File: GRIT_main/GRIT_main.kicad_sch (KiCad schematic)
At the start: 22 parts, among them J1 Raspberry_Pi_4, M1 Motor_DC, M2 Motor_DC, M3 Motor_DC, M4 Motor_DC

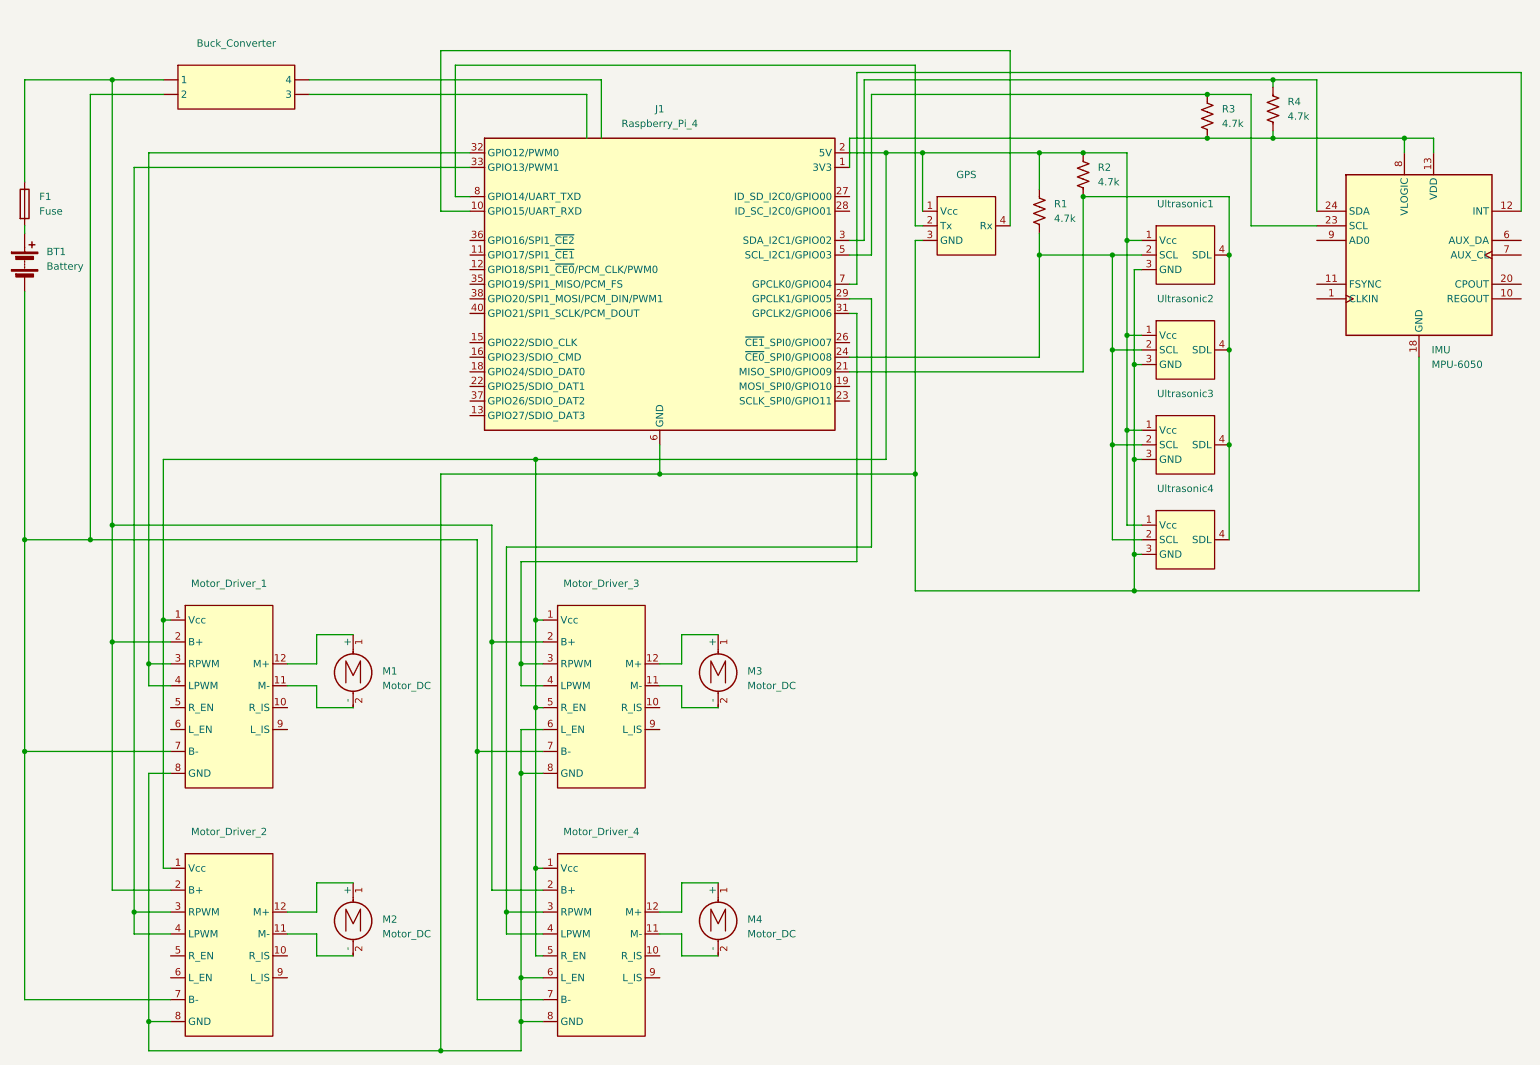
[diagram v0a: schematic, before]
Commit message: Updated Schematic
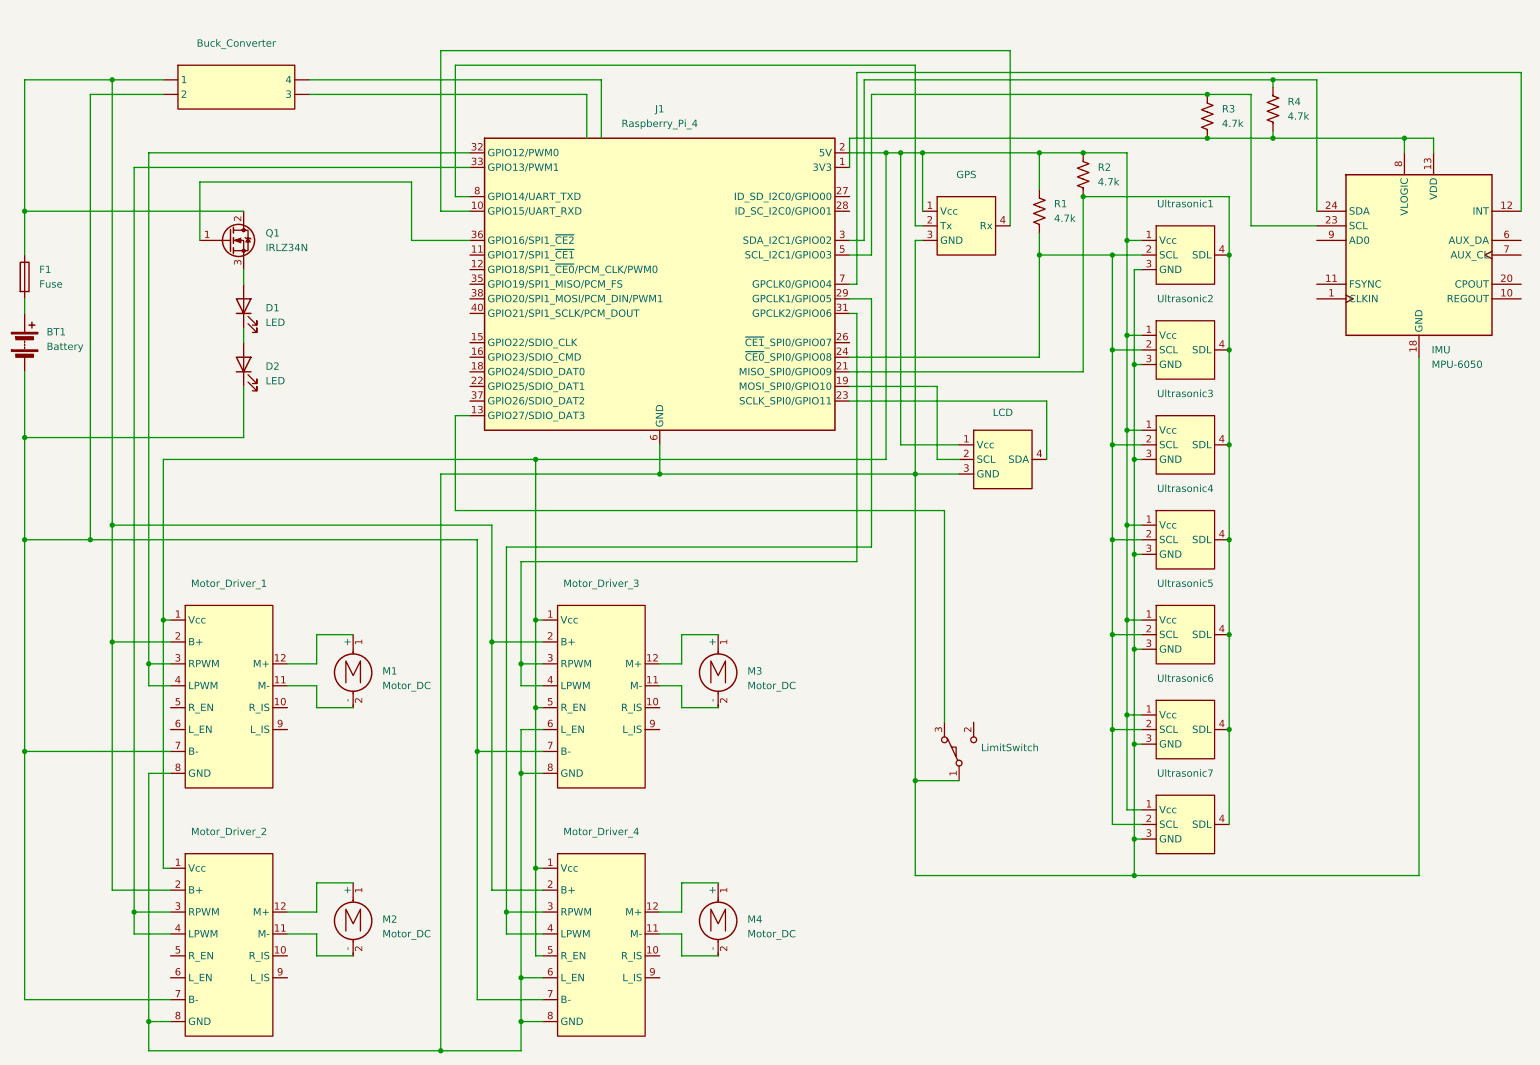
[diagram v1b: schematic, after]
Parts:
- added D1, D2: LED, symbol Device:LED
- added LCD: ~, symbol Custom_Symbols:I2C_LCD_Screen
- added LimitSwitch: ~, symbol Switch:SW_SPDT_XKB_DMx-xxxx-1
- added Q1: IRLZ34N, Package_TO_SOT_THT:TO-220-3_Vertical, symbol Transistor_FET:IRLZ34N
- added Ultrasonic5, Ultrasonic6, Ultrasonic7: ~, symbol Custom_Symbols:I2C_Ultrasonic_Sensor
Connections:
- net at GPS.3 (GND), IMU.18 (GND), J1.14 (GND)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: now also LCD.3 (GND), LimitSwitch.1 (A), Ultrasonic5.3 (GND), Ultrasonic6.3 (GND), Ultrasonic7.3 (GND)
- net at GPS.1 (Vcc), J1.2 (5V), J1.4 (5V)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: now also LCD.1 (Vcc), Ultrasonic5.1 (Vcc), Ultrasonic6.1 (Vcc), Ultrasonic7.1 (Vcc)
- net at Buck_Converter. (4), F1.1, Motor_Driver_1.2 (B+)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: now also Q1.2 (D)
- net at BT1.2 (-), Buck_Converter. (4), Motor_Driver_1.7 (B-)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: now also D2.1 (K)
- net at J1.13 (GPIO27/SDIO_DAT3): now also LimitSwitch.3 (C)
- net at J1.19 (MOSI_SPI0/GPIO10): now also LCD.2 (SCL)
- net at J1.21 (MISO_SPI0/GPIO09), R2.2, Ultrasonic1.4 (SDL)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: now also Ultrasonic5.4 (SDL), Ultrasonic6.4 (SDL), Ultrasonic7.4 (SDL)
- net at J1.23 (SCLK_SPI0/GPIO11): now also LCD.4 (SDA)
- net at J1.24 (~{CE0}_SPI0/GPIO08), R1.2, Ultrasonic1.2 (SCL)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: now also Ultrasonic5.2 (SCL), Ultrasonic6.2 (SCL), Ultrasonic7.2 (SCL)
- net at J1.36 (GPIO16/SPI1_~{CE2}): now also Q1.1 (G)
- new net: D1.2 (A), Q1.3 (S)
- new net: D1.1 (K), D2.2 (A)
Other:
- moved on the sheet: BT1, F1

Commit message: Updated Design
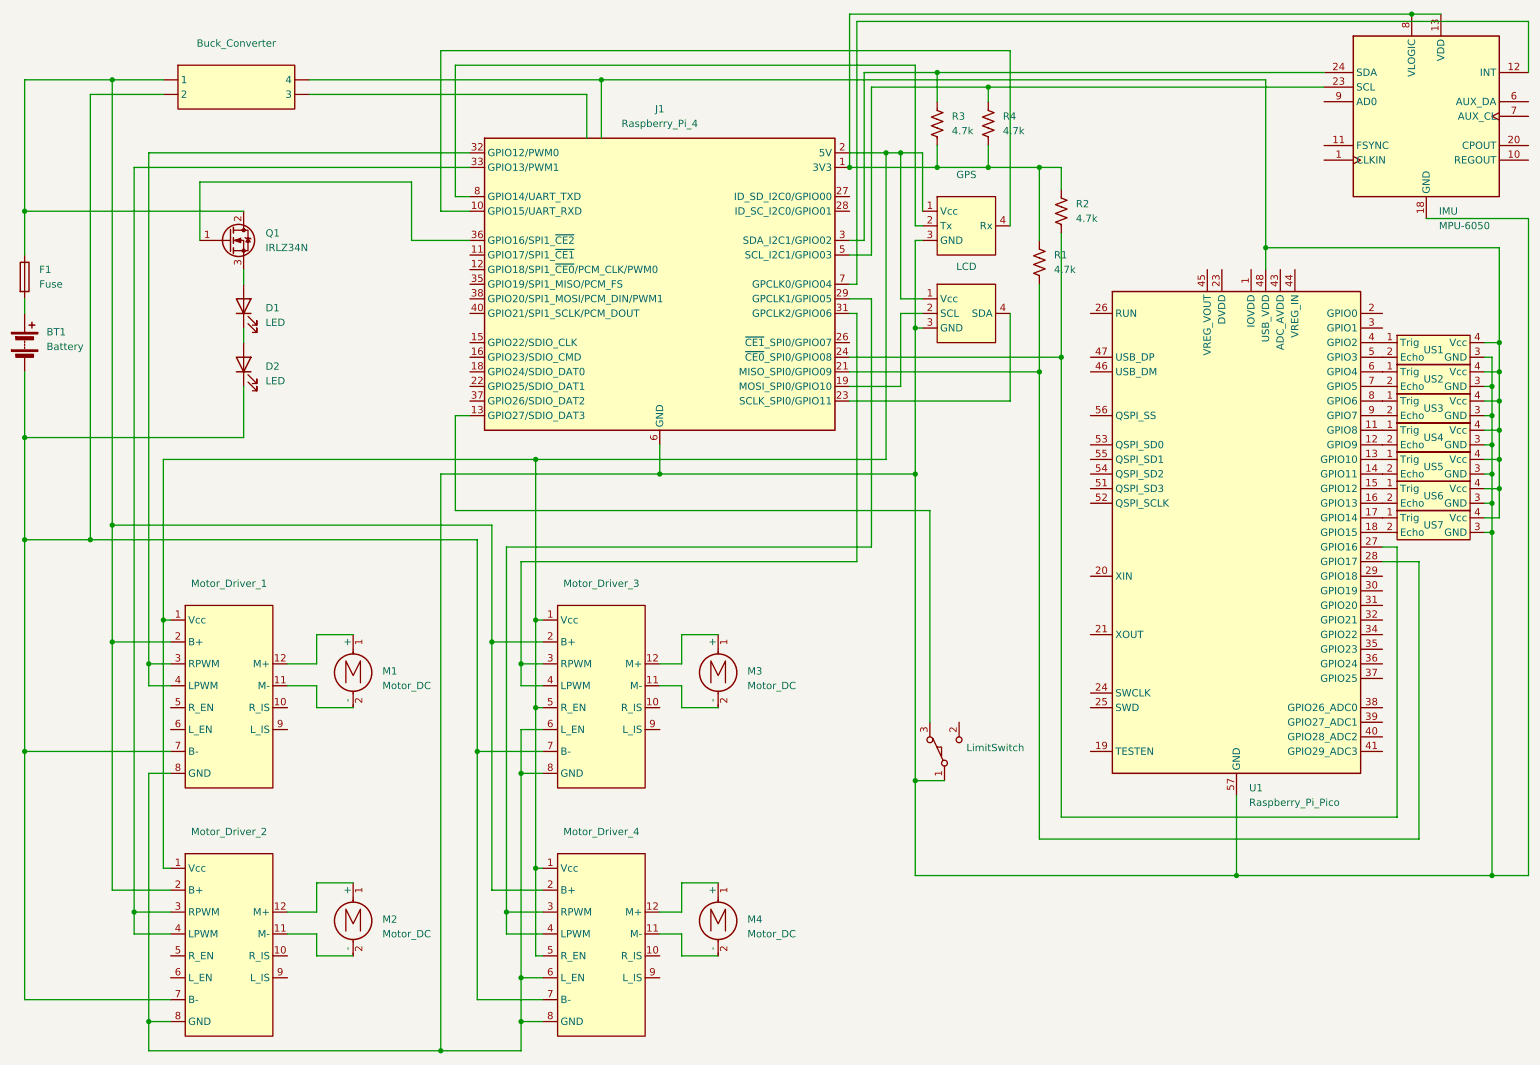
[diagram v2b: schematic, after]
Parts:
- removed Ultrasonic1, Ultrasonic2, Ultrasonic3, Ultrasonic4, Ultrasonic5, Ultrasonic6, Ultrasonic7: ~, symbol Custom_Symbols:I2C_Ultrasonic_Sensor
- added U1: Raspberry_Pi_Pico, Package_DFN_QFN:QFN-56-1EP_7x7mm_P0.4mm_EP3.2x3.2mm, symbol MCU_RaspberryPi:RP2040
- added US1, US2, US3, US4, US5, US6, US7: ~, symbol Custom_Symbols:I2C_Ultrasonic_Sensor
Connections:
- net at GPS.1 (Vcc), J1.2 (5V), J1.4 (5V)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: no longer R1.1, R2.1
- net at R1.2: now also J1.21 (MISO_SPI0/GPIO09), U1.28 (GPIO17); no longer J1.24 (~{CE0}_SPI0/GPIO08)
- net at GPS.3 (GND), IMU.18 (GND), J1.14 (GND)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: now also U1.57 (GND), US1.3 (GND), US2.3 (GND), US3.3 (GND), US4.3 (GND), US5.3 (GND), US6.3 (GND), US7.3 (GND)
- net at R2.2: now also J1.24 (~{CE0}_SPI0/GPIO08), U1.27 (GPIO16); no longer J1.21 (MISO_SPI0/GPIO09)
- net at IMU.13 (VDD), IMU.8 (VLOGIC), J1.1 (3V3)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: now also R1.1, R2.1
- net at IMU.23 (SCL), J1.5 (SCL_I2C1/GPIO03): now also R4.1; no longer R3.1
- net at IMU.24 (SDA), J1.3 (SDA_I2C1/GPIO02): now also R3.1; no longer R4.1
- new net: U1.4 (GPIO2), US1.1 (Trig)
- new net: U1.5 (GPIO3), US1.2 (Echo)
- new net: Buck_Converter. (4), U1.48 (USB_VDD), US1.4 (Vcc), US2.4 (Vcc), US3.4 (Vcc), US4.4 (Vcc), US5.4 (Vcc), US6.4 (Vcc), US7.4 (Vcc)
- new net: U1.15 (GPIO12), US6.1 (Trig)
- new net: U1.16 (GPIO13), US6.2 (Echo)
- new net: U1.6 (GPIO4), US2.1 (Trig)
- new net: U1.7 (GPIO5), US2.2 (Echo)
- new net: U1.17 (GPIO14), US7.1 (Trig)
- new net: U1.18 (GPIO15), US7.2 (Echo)
- new net: U1.11 (GPIO8), US4.1 (Trig)
- new net: U1.12 (GPIO9), US4.2 (Echo)
- new net: U1.8 (GPIO6), US3.1 (Trig)
- new net: U1.9 (GPIO7), US3.2 (Echo)
- new net: U1.1 (IOVDD), U1.10 (IOVDD), U1.22 (IOVDD), U1.33 (IOVDD), U1.42 (IOVDD), U1.49 (IOVDD)
- new net: U1.13 (GPIO10), US5.1 (Trig)
- new net: U1.14 (GPIO11), US5.2 (Echo)
- new net: U1.23 (DVDD), U1.50 (DVDD)
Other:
- moved on the sheet: IMU, LCD, LimitSwitch
